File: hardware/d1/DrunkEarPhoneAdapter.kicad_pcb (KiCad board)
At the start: 2 copper layers, 40.3 x 34.7 mm, 9 parts, among them U1 CS43131-CNZR, U2 STM32G0B1VCT6, U4 TCPP03-M20, U5 TCPP03-M20, U6 ES8327, X1 X322516MLB4SI, X2 OT7EL89CJI-111YLC-24_576M

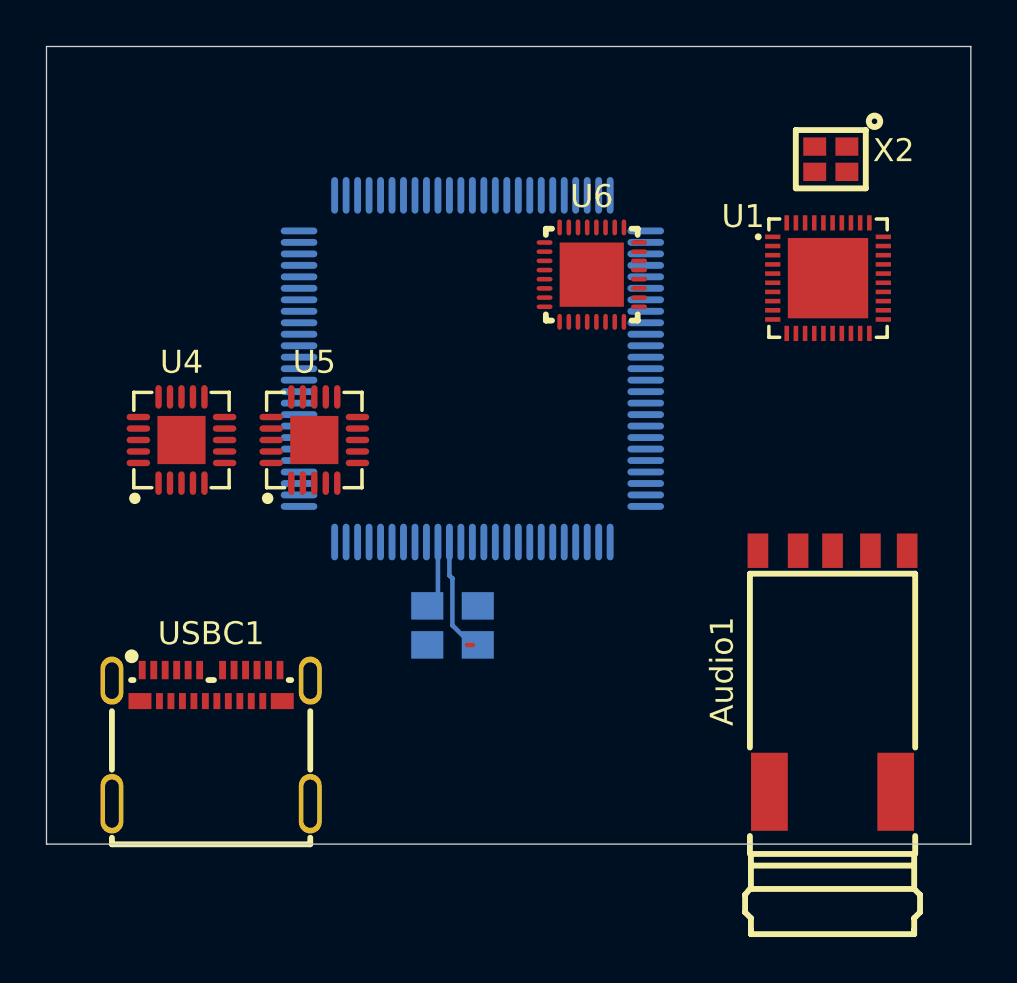
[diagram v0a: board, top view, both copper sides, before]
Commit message: New components
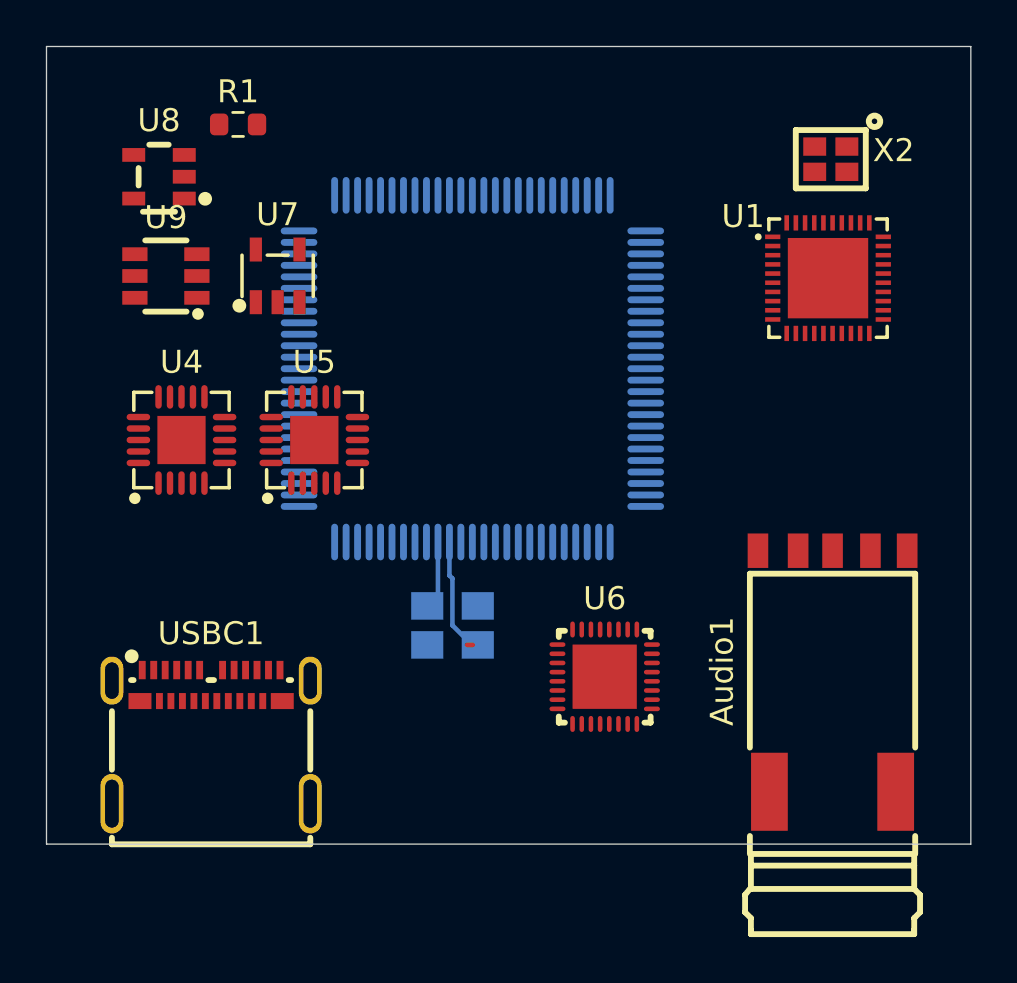
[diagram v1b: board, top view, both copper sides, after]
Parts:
- added R1: 10k, Resistor_SMD:R_0603_1608Metric, F.Cu at (28.3, 24.2)
- added U7: TPS7A2018PDBVR, JLCImport:TPS7A2018PDBVR, F.Cu at (30.1, 30.8)
- added U8: TPS7A2033PDBVR, JLCImport:TPS7A2033PDBVR, F.Cu at (24.9, 26.5)
- added U9: TPS560430XFDBVR, JLCImport:TPS560430XFDBVR, F.Cu at (25.2, 30.8)
- moved U6 17.5 mm to (44.3, 48.3)
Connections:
- U1 pad 38: unconnected-(U1-LRCK1-Pad38) -> /dac/I2S_WS
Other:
- copper layers 2 -> 4
